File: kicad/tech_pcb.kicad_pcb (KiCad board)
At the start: 2 copper layers, 22.4 x 34 mm, 24 parts, among them J1 Conn_01x11, J2 Conn_01x11, J3 USB_C_Receptacle_USB2.0_16P, J4 Conn_01x03_MountingPin, SW1 RST, SW2 BOOT, U1 STM32C071GBUxN, U2 XC6206PxxxMR

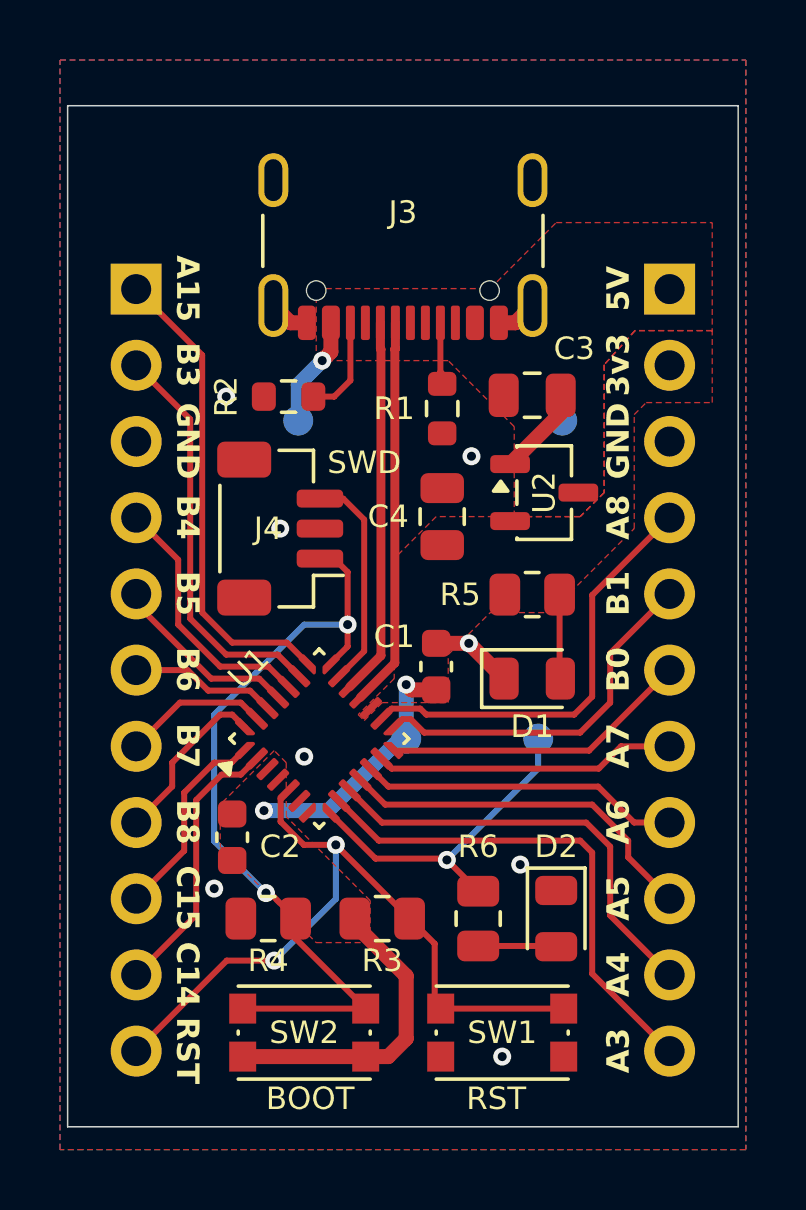
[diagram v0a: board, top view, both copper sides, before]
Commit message: Forgot to run DRC
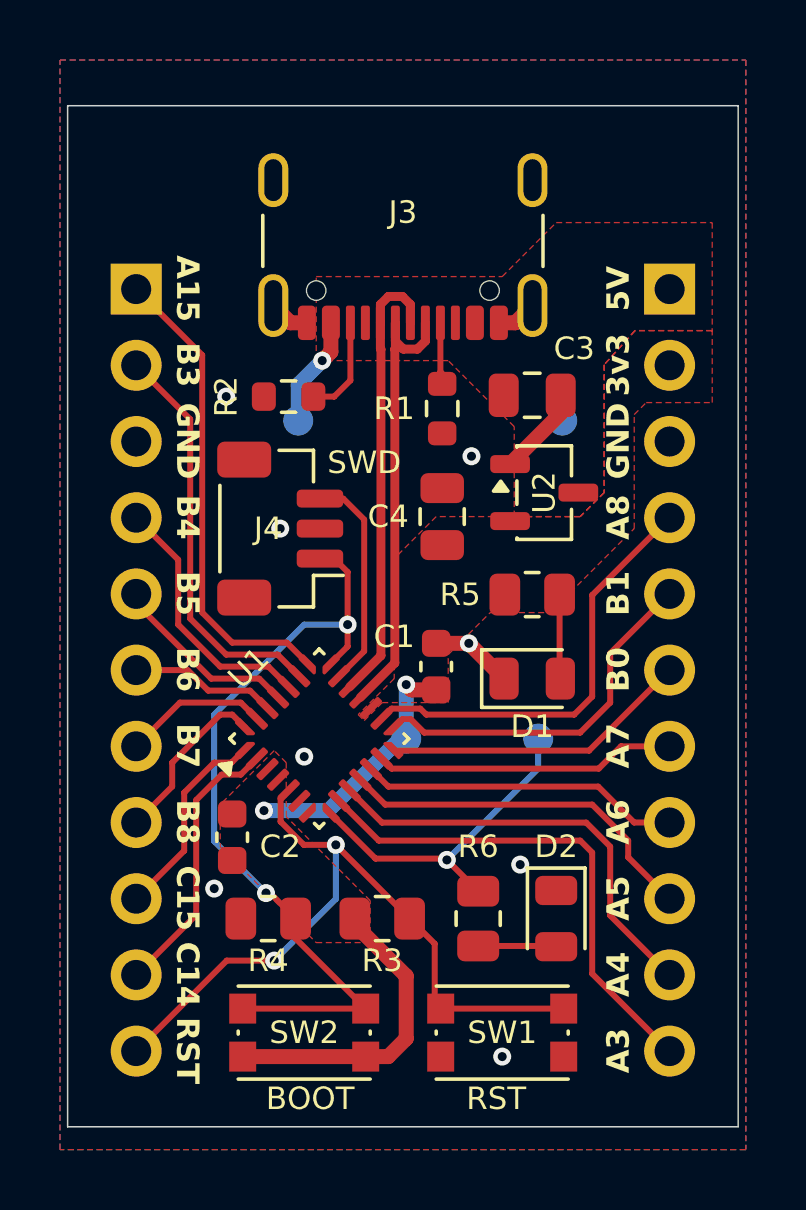
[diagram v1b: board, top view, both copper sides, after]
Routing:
- net /USB_DN: track 13.0 -> 15.4 mm
- net /USB_DP: track 12.6 -> 15.0 mm
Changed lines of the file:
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@@
+	)
+	(segment
+		(start 33.806596 25.6626)
+		(end 34.273404 25.6626)
+		(width 0.3)
+		(layer "F.Cu")
+		(net "/USB_DP")
 	)
 	(segment
@@
 	)
 	(segment
+		(start 33.54 25.929196)
+		(end 33.806596 25.6626)
+		(width 0.3)
+		(layer "F.Cu")
+		(net "/USB_DP")
+	)
+	(segment
+		(start 33.54 26.54)
+		(end 33.54 25.929196)
+		(width 0.3)
+		(layer "F.Cu")
+		(net "/USB_DP")
+	)
+	(segment
 		(start 33.55875 27.421251)
 		(end 33.54 27.402501)
@@
 	)
 	(segment
+		(start 34.273404 25.6626)
+		(end 34.54 25.929196)
+		(width 0.3)
+		(layer "F.Cu")
+		(net "/USB_DP")
+	)
+	(segment
+		(start 34.54 25.929196)
+		(end 34.54 26.54)
+		(width 0.3)
+		(layer "F.Cu")
+		(net "/USB_DP")
+	)
+	(segment
 		(start 32.516466 38.676427)
 		(end 33.55875 37.634143)
@@
 	)
 	(segment
+		(start 34.04 27.150804)
+		(end 34.04 26.54)
+		(width 0.3)
+		(layer "F.Cu")
+		(net "/USB_DN")
+	)
+	(segment
+		(start 34.773404 27.4174)
+		(end 34.306596 27.4174)
+		(width 0.3)
+		(layer "F.Cu")
+		(net "/USB_DN")
+	)
+	(segment
 		(start 34.02125 37.87875)
 		(end 34.02125 27.421251)
@@
 		(start 34.04 27.402501)
 		(end 34.04 26.54)
+		(width 0.3)
+		(layer "F.Cu")
+		(net "/USB_DN")
+	)
+	(segment
+		(start 35.04 27.150804)
+		(end 34.773404 27.4174)
+		(width 0.3)
+		(layer "F.Cu")
+		(net "/USB_DN")
+	)
+	(segment
+		(start 34.306596 27.4174)
+		(end 34.04 27.150804)
+		(width 0.3)
+		(layer "F.Cu")
+		(net "/USB_DN")
+	)
+	(segment
+		(start 35.04 26.54)
+		(end 35.04 27.150804)
 		(width 0.3)
 		(layer "F.Cu")
@@
 		(polygon
 			(pts
-				(xy 31.4 27.8) (xy 31.4 25.4) (xy 37.2 25.4) (xy 39.4 23.2) (xy 44.6 23.2) (xy 44.6 26.8) (xy 42.036364 26.8)
+				(xy 31.4 27.8) (xy 31.4 25) (xy 37.6 25) (xy 39.4 23.2) (xy 44.6 23.2) (xy 44.6 26.8) (xy 42.036364 26.8)
 				(xy 41 27.94) (xy 41 32.2) (xy 40.2 33) (xy 38 33) (xy 38 30) (xy 35.8 27.8)
 			)

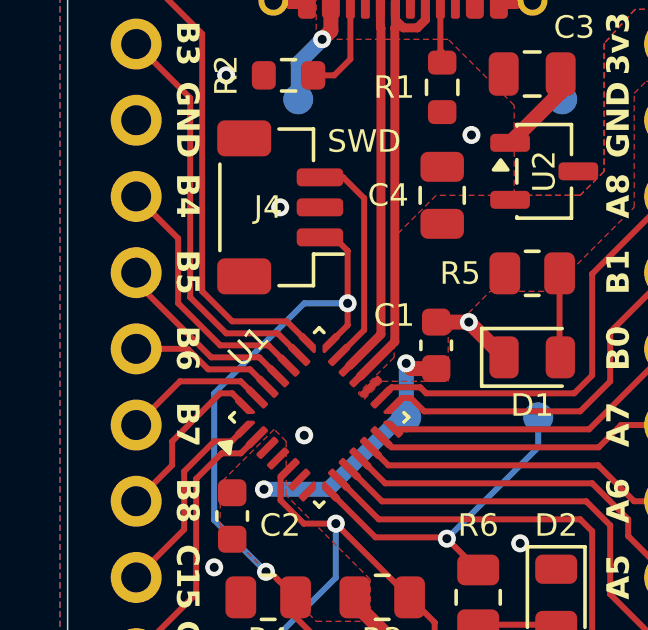
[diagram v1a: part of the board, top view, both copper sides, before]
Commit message: Tidy up the schematic
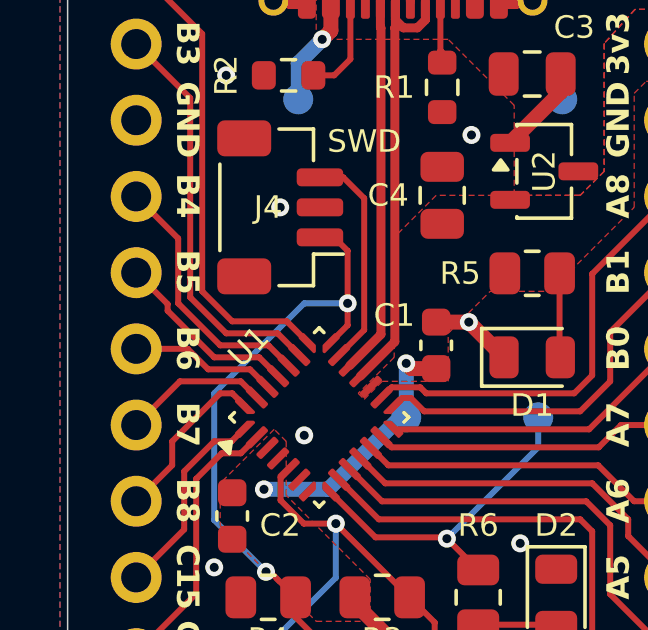
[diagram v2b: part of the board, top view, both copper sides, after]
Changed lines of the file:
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@@
 	)
 	(segment
-		(start 27.2 36.4)
-		(end 27.2 29.757)
+		(start 27.2 29.757)
+		(end 25.4 27.957)
+		(width 0.2)
+		(layer "F.Cu")
+		(net "/PB3")
+	)
+	(segment
+		(start 30.837087 38.322874)
+		(end 30.114213 37.6)
 		(width 0.2)
 		(layer "F.Cu")
@@
 	)
 	(segment
+		(start 27.2 36.4)
+		(end 27.2 29.757)
+		(width 0.2)
+		(layer "F.Cu")
+		(net "/PB3")
+	)
+	(segment
 		(start 28.4 37.6)
 		(end 27.2 36.4)
@@
 	)
 	(segment
-		(start 30.837087 38.322874)
-		(end 30.114213 37.6)
+		(start 30.483534 38.676427)
+		(end 29.807107 38)
 		(width 0.2)
 		(layer "F.Cu")
-		(net "/PB3")
+		(net "/PB4")
 	)
 	(segment
-		(start 27.2 29.757)
-		(end 25.4 27.957)
-		(width 0.2)
-		(layer "F.Cu")
-		(net "/PB3")
-	)
-	(segment
-		(start 26.8 36.6)
-		(end 26.8 34.437)
+		(start 28.2 38)
+		(end 26.8 36.6)
 		(width 0.2)
 		(layer "F.Cu")
@@
 	)
 	(segment
+		(start 26.8 36.6)
+		(end 26.8 34.437)
+		(width 0.2)
+		(layer "F.Cu")
+		(net "/PB4")
+	)
+	(segment
 		(start 29.807107 38)
 		(end 28.2 38)
@@
 	)
 	(segment
-		(start 28.2 38)
-		(end 26.8 36.6)
-		(width 0.2)
-		(layer "F.Cu")
-		(net "/PB4")
-	)
-	(segment
-		(start 30.483534 38.676427)
-		(end 29.807107 38)
-		(width 0.2)
-		(layer "F.Cu")
-		(net "/PB4")
-	)
-	(segment
-		(start 29.5 38.4)
-		(end 27.9 38.4)
+		(start 30.129981 39.029981)
+		(end 29.5 38.4)
 		(width 0.2)
 		(layer "F.Cu")
@@
 	)
 	(segment
-		(start 25.4 35.9)
-		(end 25.4 35.577)
+		(start 26.4476 36.8476)
+		(end 26.4476 36.6246)
 		(width 0.2)
 		(layer "F.Cu")
@@
 	)
 	(segment
-		(start 27.9 38.4)
-		(end 25.4 35.9)
+		(start 28 38.4)
+		(end 26.4476 36.8476)
 		(width 0.2)
 		(layer "F.Cu")
@@
 	)
 	(segment
-		(start 30.129981 39.029981)
-		(end 29.5 38.4)
+		(start 29.5 38.4)
+		(end 28 38.4)
 		(width 0.2)
 		(layer "F.Cu")
+		(net "/PB5")
+	)
+	(segment
+		(start 26.4476 36.6246)
+		(end 25.4 35.577)
+		(width 0.2)
+		(layer "F.Cu")
